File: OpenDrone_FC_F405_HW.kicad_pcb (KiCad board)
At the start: 2 copper layers, 34 x 34 mm, 79 parts, among them J1 Conn_01x05, J10 Conn_01x06, J11 Conn_01x06, J12 Conn_01x06, J17 Conn_02x03_Odd_Even, J6 Conn_01x08, J8 Conn_01x04, U1 STM32F405RGTx, U2 TPS54331, U3 ICM42688, U5 HMC5883L, U6 BMP280, U7 TPS54331, U8 Board, Y2 8Mhz

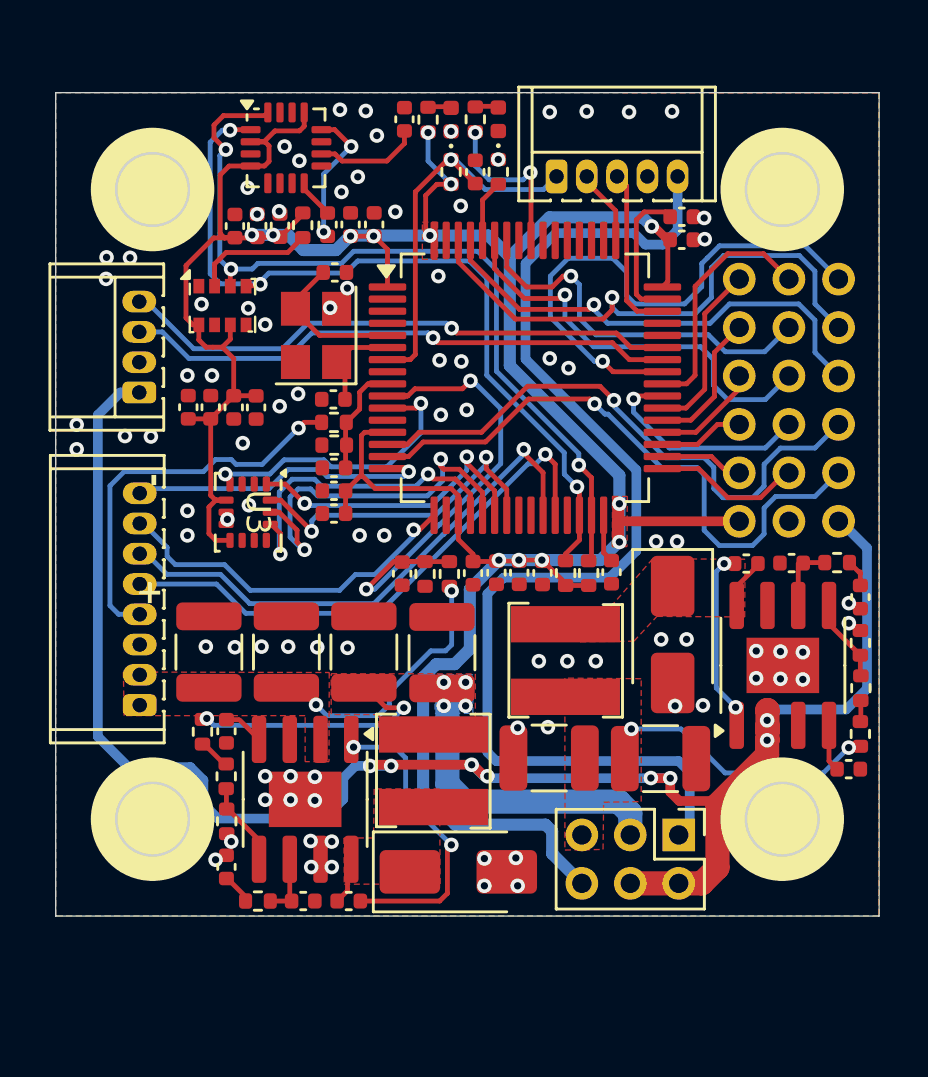
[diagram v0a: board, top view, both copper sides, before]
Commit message: update setting
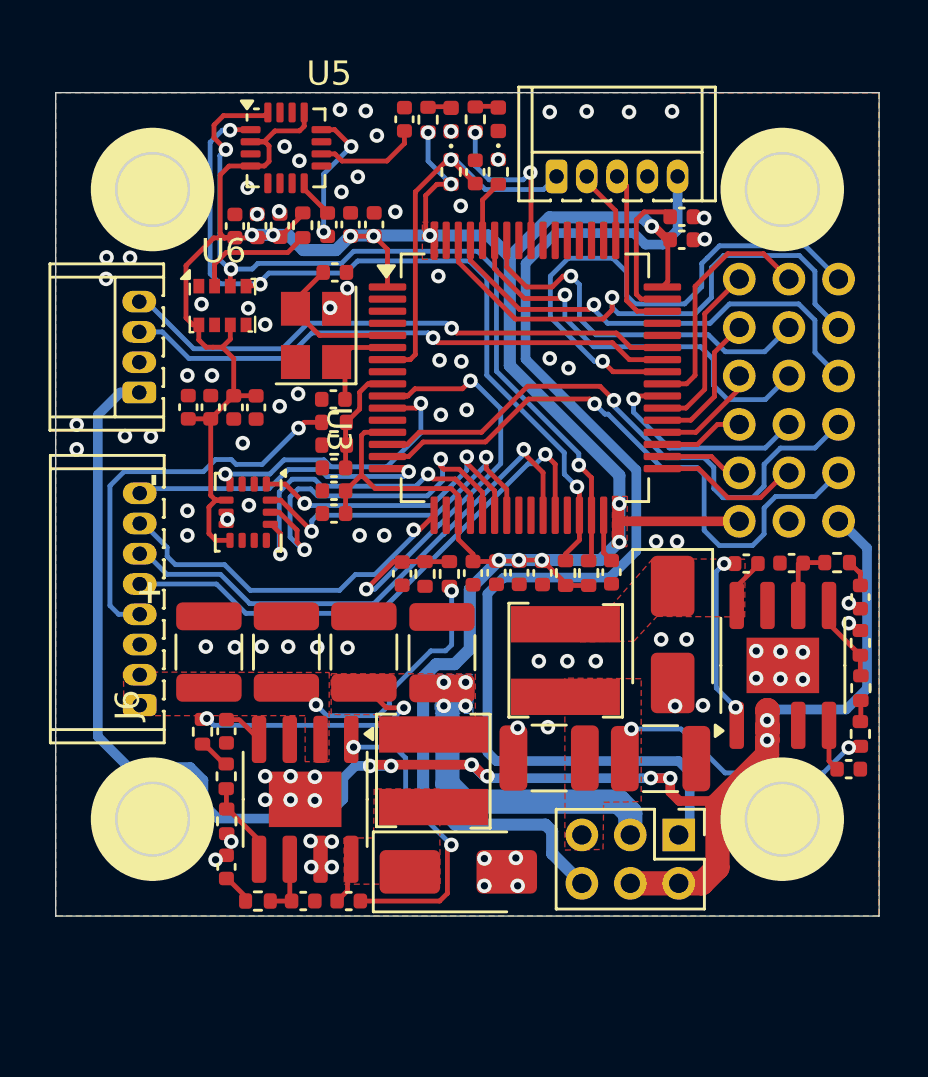
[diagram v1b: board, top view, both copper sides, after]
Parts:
- J6: footprint Footprint:Connector_XH_1x08_P1.25mm_Horizontal -> KiCad-Lib:Connector_XH_1x08_P1.25mm_Horizontal
- U3: footprint Footprint:LGA-14_3x2.5mm_P0.5mm -> KiCad-Lib:LGA-14_3x2.5mm_P0.5mm
- U5: footprint Footprint:QFN-16_3x3mm_P0.5mm -> KiCad-Lib:QFN-16_3x3mm_P0.5mm
- U6: footprint Footprint:LGA-8_2x2.5mm_P0.65mm -> KiCad-Lib:LGA-8_2x2.5mm_P0.65mm
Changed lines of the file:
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@@
 		(tags "capacitor")
 		(property "Reference" "C13"
-			(at 0 -1.16 360)
+			(at 0 -1.16 0)
 			(layer "B.SilkS")
 			(hide yes)
@@
 		)
 		(property "Value" "10nF"
-			(at 0 1.16 360)
+			(at 0 1.16 0)
 			(layer "F.Fab")
 			(hide yes)
@@
 		)
 		(fp_text user "${REFERENCE}"
-			(at 0 0 360)
+			(at 0 0 0)
 			(layer "F.Fab")
 			(effects
@@
 		)
 	)
-	(footprint "Footprint:QFN-16_3x3mm_P0.5mm"
+	(footprint "KiCad-Lib:QFN-16_3x3mm_P0.5mm"
 		(layer "F.Cu")
 		(at 143.01 68.58)
 		(property "Reference" "U5"
-			(at 0 -0.5 0)
+			(at 1.78 -3.07 0)
 			(unlocked yes)
-			(layer "B.SilkS")
-			(hide yes)
+			(layer "F.SilkS")
 			(effects
 				(font
@@
 			(unlocked yes)
 			(layer "F.Fab")
-			(hide yes)
 			(effects
 				(font
@@
 			)
 		)
-		(property "Footprint" "Footprint:QFN-16_3x3mm_P0.5mm"
+		(property "Footprint" "KiCad-Lib:QFN-16_3x3mm_P0.5mm"
 			(at 0 0 0)
 			(unlocked yes)
@@
 		)
 	)
-	(footprint "Footprint:LGA-14_3x2.5mm_P0.5mm"
+	(footprint "KiCad-Lib:LGA-14_3x2.5mm_P0.5mm"
 		(layer "F.Cu")
 		(at 141.45 83.625 -90)
 		(property "Reference" "U3"
-			(at 0 -0.4 -90)
+			(at -3.43 -3.74 -90)
 			(unlocked yes)
 			(layer "F.SilkS")
@@
 			)
 		)
-		(property "Footprint" "Footprint:LGA-14_3x2.5mm_P0.5mm"
+		(property "Footprint" "KiCad-Lib:LGA-14_3x2.5mm_P0.5mm"
 			(at 0 0.09 -90)
 			(unlocked yes)
@@
 		)
 	)
-	(footprint "Footprint:Connector_XH_1x08_P1.25mm_Horizontal"
+	(footprint "KiCad-Lib:Connector_XH_1x08_P1.25mm_Horizontal"
 		(layer "F.Cu")
 		(at 136.97 91.59 90)
@@
 			(at 0 -0.5 90)
 			(unlocked yes)
-			(layer "B.SilkS")
-			(hide yes)
+			(layer "F.SilkS")
 			(effects
 				(font
@@
 			(unlocked yes)
 			(layer "F.Fab")
-			(hide yes)
 			(effects
 				(font
@@
 			)
 		)
-		(property "Footprint" "Footprint:Connector_XH_1x08_P1.25mm_Horizontal"
+		(property "Footprint" "KiCad-Lib:Connector_XH_1x08_P1.25mm_Horizontal"
 			(at 0 0 90)
 			(unlocked yes)
@@
 		)
 		(fp_text user "${REFERENCE}"
-			(at 3.62 2.39 0)
-			(unlocked yes)
+			(at 4.38 -3.8 90)
 			(layer "F.Fab")
 			(effects
@@
 		)
 		(fp_text user "${REFERENCE}"
-			(at 4.38 -3.8 90)
+			(at 0 2.5 90)
+			(unlocked yes)
 			(layer "F.Fab")
 			(effects
@@
 		)
 	)
-	(footprint "Footprint:LGA-8_2x2.5mm_P0.65mm"
+	(footprint "KiCad-Lib:LGA-8_2x2.5mm_P0.65mm"
 		(layer "F.Cu")
 		(at 140.39 75.1)
 		(property "Reference" "U6"
-			(at 0 -0.5 0)
+			(at 0.04 -2.26 0)
 			(unlocked yes)
-			(layer "B.SilkS")
-			(hide yes)
+			(layer "F.SilkS")
 			(effects
 				(font
@@
 			(unlocked yes)
 			(layer "F.Fab")
-			(hide yes)
 			(effects
 				(font
@@
 			)
 		)
-		(property "Footprint" "Footprint:LGA-8_2x2.5mm_P0.65mm"
-			(at 0 0 0)
+		(property "Footprint" "KiCad-Lib:LGA-8_2x2.5mm_P0.65mm"
+			(at -1.56 1.31 0)
 			(unlocked yes)
 			(layer "F.Fab")
@@
 		)
 		(property "Datasheet" "https://ae-bst.resource.bosch.com/media/_tech/media/datasheets/BST-BMP280-DS001.pdf"
-			(at 0 0 0)
+			(at -1.56 1.31 0)
 			(unlocked yes)
 			(layer "F.Fab")
@@
 		)
 		(property "Description" "Absolute Barometric Pressure Sensor, LGA-8"
-			(at 0 0 0)
+			(at -1.56 1.31 0)
 			(unlocked yes)
 			(layer "F.Fab")

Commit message: update
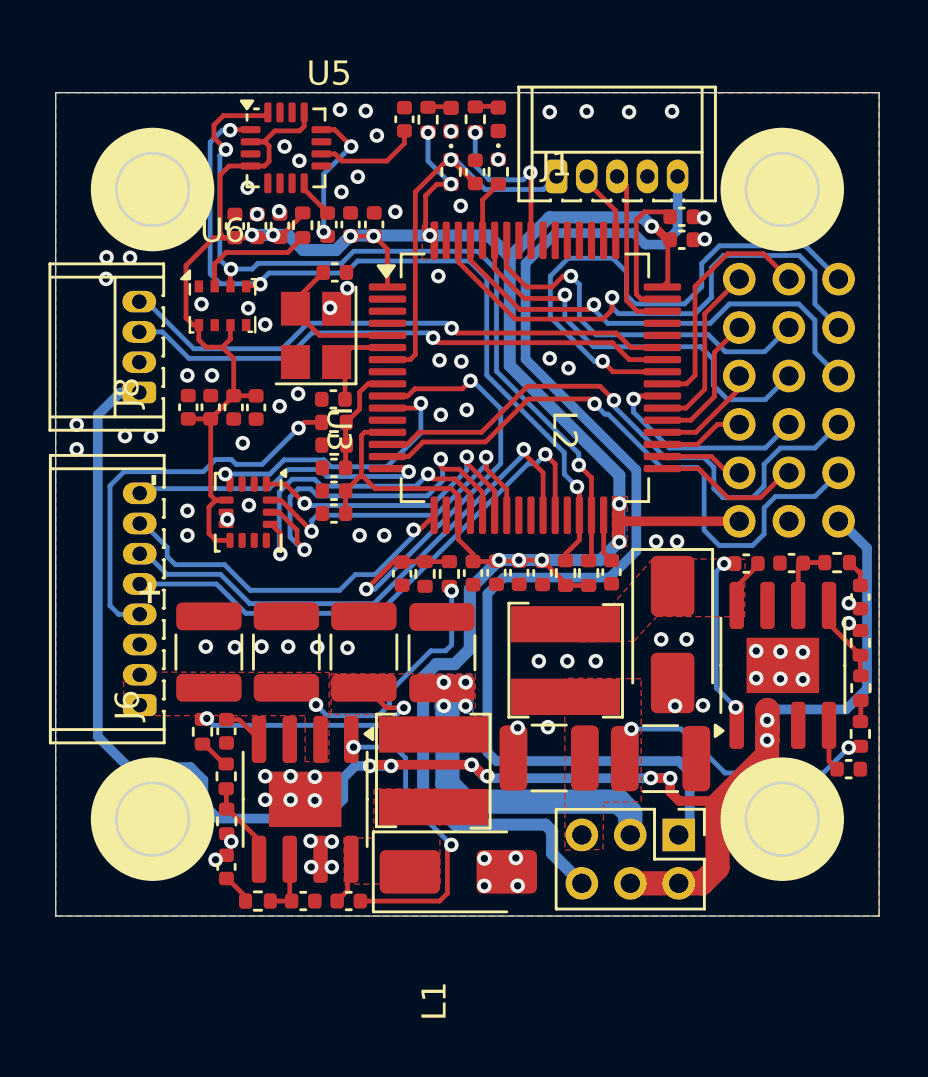
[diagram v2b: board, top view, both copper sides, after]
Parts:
- J1: footprint Footprint:Connector_XH_1x05_P1.25mm_Horizontal -> KiCad-Lib:Connector_XH_1x05_P1.25mm_Horizontal
- J10, J11, J12: footprint Footprint:Header_1x06_P2.00mm_Vertical -> KiCad-Lib:Header_1x06_P2.00mm_Vertical
- J8: footprint Footprint:Connector_XH_1x04_P1.25mm_Horizontal -> KiCad-Lib:Connector_XH_1x04_P1.25mm_Horizontal
- L1, L2: footprint Footprint:Inductor_SMD_4D28 -> KiCad-Lib:Inductor_SMD_4D28
- U6: footprint KiCad-Lib:LGA-8_2x2.5mm_P0.65mm -> Package_LGA:Bosch_LGA-8_2x2.5mm_P0.65mm_ClockwisePinNumbering
- U8: footprint Footprint:Board_Outline_34x34_Hole_26x26 -> Proj-Lib:Board_Outline_34x34_Hole_26x26
